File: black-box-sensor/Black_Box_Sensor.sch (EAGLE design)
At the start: 65 parts, among them J1 104031-0811, J2 UX60-MB-5S8, J3 B4B-PH-SM4-TBT(LF)(SN), U1 ADXL375, U2 ADXL375, U3 ATMEGA32U4-AU, U4 ATSAMD21G17A-AU, U5 IAM-20380, U6 NL27WZ32USG, U7 LT1129CST-5#PBF, U8 AD8426ACPZ-WP, U9 TXU0304

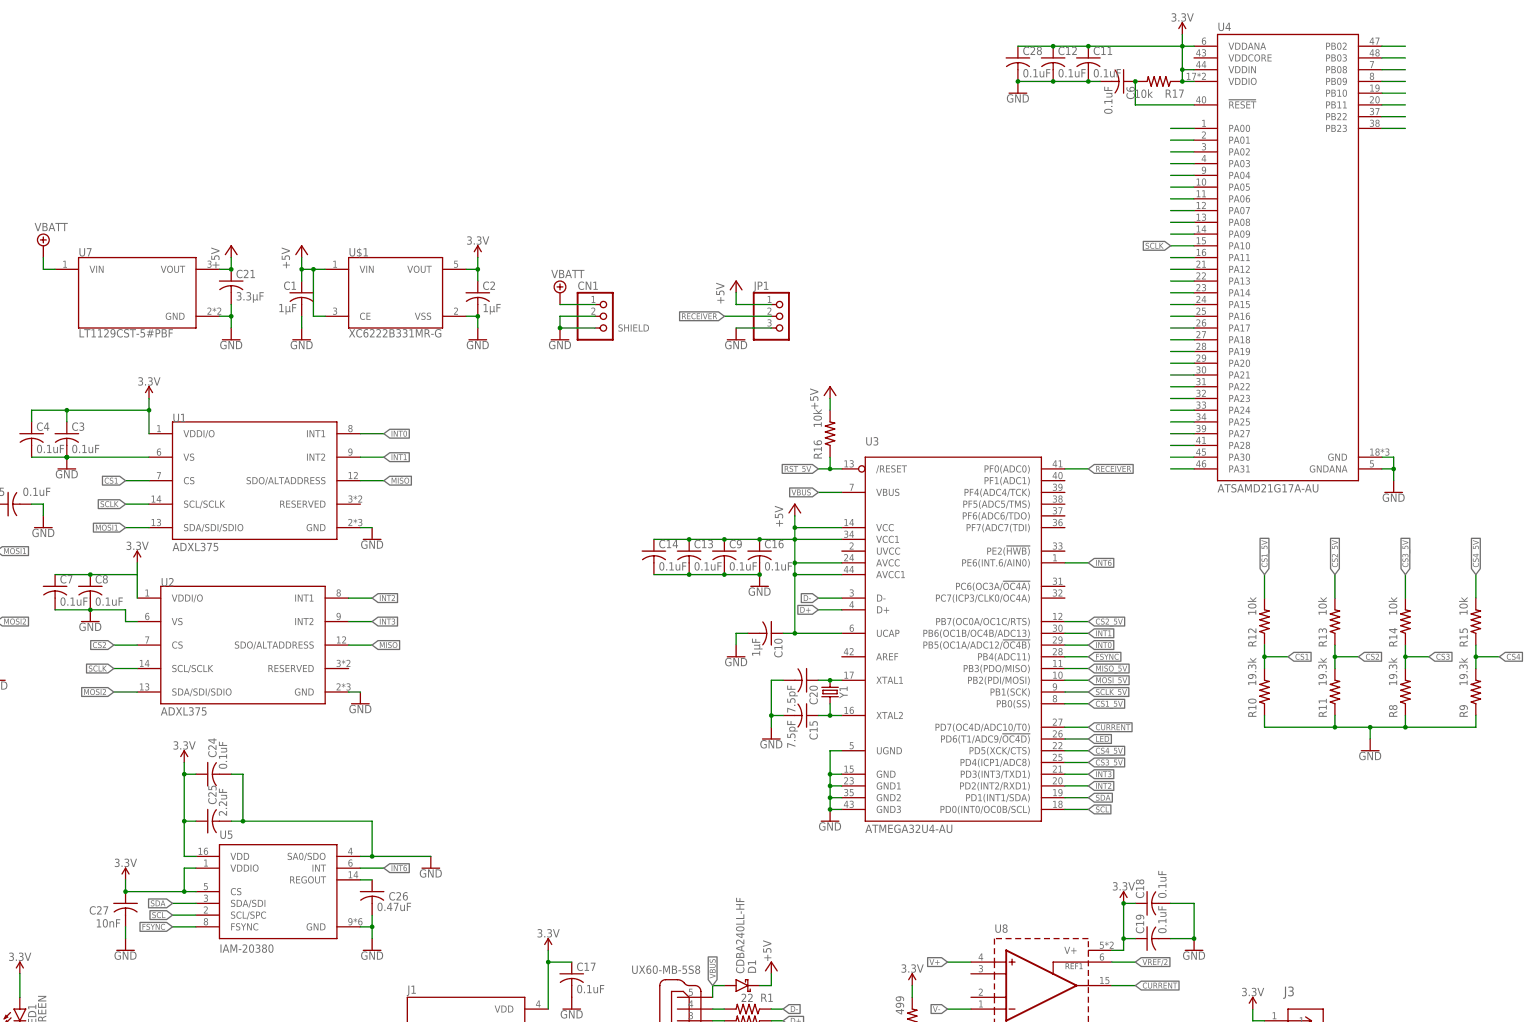
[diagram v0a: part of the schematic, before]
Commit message: finalize for review
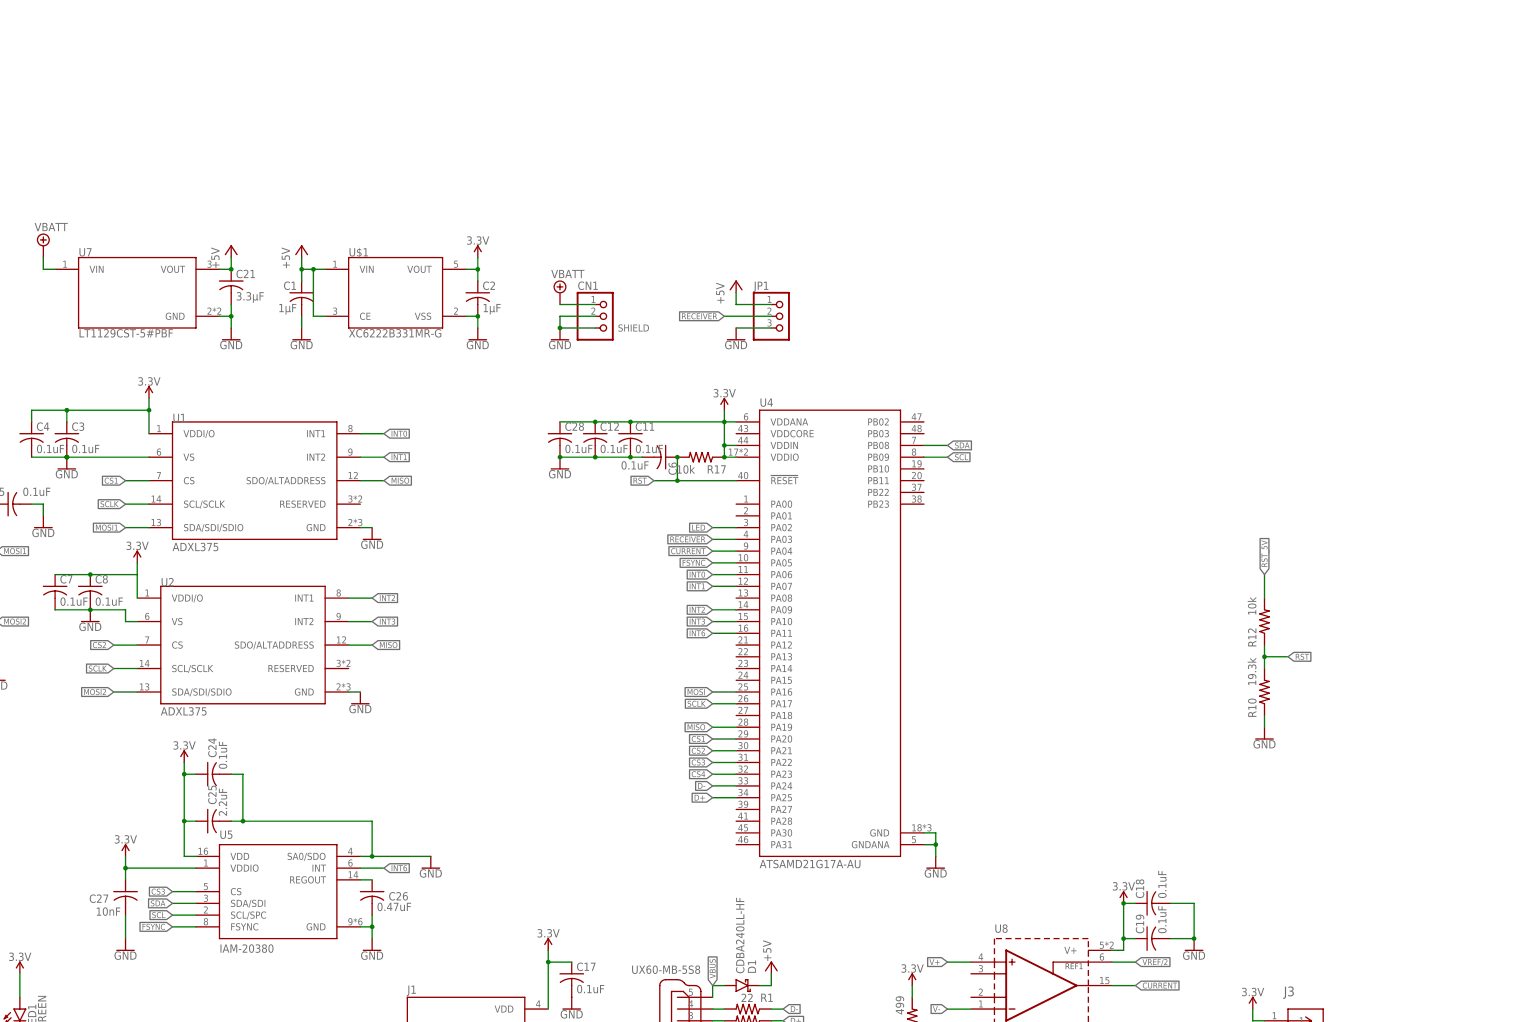
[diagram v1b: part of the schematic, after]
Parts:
- removed C10: 1µF, rcl:C-USC0603
- removed C13, C14, C16, C9: 0.1uF, rcl:C-USC0603
- removed C15, C20: 7.5pF, rcl:C-USC0603
- removed R11, R8, R9: 19.3k, rcl:R-US_R0603
- removed R13, R14, R15, R16: 10k, rcl:R-US_R0603
- removed U3: ATMEGA32U4-AU, BBS_Library:ATMEGA32U4-AU
- removed Y1: (no value), SparkFun-Clocks:CRYSTALSMD-3.2X2.5
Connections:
- removed net CS1_5V: R12.2, U3.PB0(SS)
- removed net CS2_5V: R13.2, U3.PB7(OC0A/OC1C/RTS)
- removed net CS3_5V: R14.2, U3.PD4(ICP1/ADC8)
- removed net CS4_5V: R15.2, U3.PD5(XCK/CTS)
- removed net N$14: C6.1, R17.2, U4.!RESET!
- removed net N$15: U4.PA00
- removed net N$16: U4.PA01
- removed net N$17: U4.PA02
- removed net N$18: U4.PA03
- removed net N$19: U4.PA04
- removed net N$20: U4.PA05
- removed net N$21: U4.PA06
- removed net N$22: U4.PA07
- removed net N$23: U4.PA08
- removed net N$24: U4.PA09
- removed net N$26: U4.PA11
- removed net N$27: U4.PA12
- removed net N$28: U4.PA13
- removed net N$29: U4.PA14
- removed net N$30: U4.PA15
- removed net N$31: U4.PA16
- removed net N$32: U4.PA17
- removed net N$33: U4.PA18
- removed net N$34: U4.PA19
- removed net N$35: U4.PA20
- removed net N$36: U4.PA21
- removed net N$37: U4.PA22
- removed net N$38: U4.PA23
- removed net N$39: U4.PA24
- removed net N$40: U4.PA25
- removed net N$41: U4.PA27
- removed net N$42: U4.PA28
- removed net N$43: U4.PA30
- removed net N$44: U4.PA31
- removed net N$45: U4.PB02
- removed net N$46: U4.PB03
- removed net N$47: U4.PB08
- removed net N$48: U4.PB09
- removed net N$49: U4.PB10
- removed net N$50: U4.PB11
- removed net N$51: U4.PB22
- removed net N$52: U4.PB23
- removed net N$7: C15.1, U3.XTAL2, Y1.2
- removed net XTAL1: C20.1, U3.XTAL1, Y1.1
- new net RST: C6.1, R10.2, R12.1, R17.2, U4.!RESET!
- net +5V: no longer C10.1, C13.1, C14.1, C16.1, C9.1, R16.2, U3.AVCC, U3.AVCC1, U3.UCAP, U3.VCC, U3.VCC1
- net 3.3V: no longer U5.CS
- net CS1: now also U4.PA20; no longer R10.2, R12.1
- net CS2: now also U4.PA21; no longer R11.2, R13.1
- net CS3: now also U4.PA22, U5.CS; no longer R14.1, R8.2
- net CS4: now also U4.PA23; no longer R15.1, R9.2
- net CURRENT: now also U4.PA04; no longer U3.PD7(OC4D/ADC10/T0)
- net D+: now also U4.PA25; no longer U3.D+
- net D-: now also U4.PA24; no longer U3.D-
- net FSYNC: now also U4.PA05; no longer U3.PB4(ADC11)
- net GND: no longer C10.2, C13.2, C14.2, C15.2, C16.2, C20.2, C9.2, R11.1, R8.1, R9.1, U3.GND, U3.GND1, U3.GND2, U3.GND3, U3.UGND
- net INT0: now also U4.PA06; no longer U3.PB5(OC1A/ADC12/!OC4B)
- net INT1: now also U4.PA07; no longer U3.PB6(OC1B/OC4B/ADC13)
- net INT2: now also U4.PA09; no longer U3.PD2(INT2/RXD1)
- net INT3: now also U4.PA10; no longer U3.PD3(INT3/TXD1)
- net INT6: now also U4.PA11; no longer U3.PE6(INT.6/AIN0)
- net LED: now also U4.PA02; no longer U3.PD6(T1/ADC9/!OC4D)
- net MISO: now also U4.PA19
- net MISO_5V: no longer U3.PB3(PDO/MISO)
- net MOSI: now also U4.PA16
- net MOSI_5V: no longer U3.PB2(PDI/MOSI)
- net RECEIVER: now also U4.PA03; no longer U3.PF0(ADC0)
- net RST_5V: now also R12.2; no longer R16.1, U3./RESET
- net SCL: now also U4.PB09; no longer U3.PD0(INT0/OC0B/SCL)
- net SCLK: now also U4.PA17; no longer U4.PA10
- net SCLK_5V: no longer U3.PB1(SCK)
- net SDA: now also U4.PB08; no longer U3.PD1(INT1/SDA)
- net VBUS: no longer U3.VBUS
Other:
- moved on the sheet: C11, C12, C27, C28, C6, R17, U4
